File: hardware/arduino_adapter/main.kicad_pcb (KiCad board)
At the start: 2 copper layers, 65.5 x 62.5 mm, 15 parts, among them P1 CONN_8, P10 CONN_10, P11 CONN_8, P2 CONN_6, P3 CONN_6, P4 CONN_8, P5 POW, P6 TWI, P7 TWI_POW, P8 CONN_10, P9 CONN_8

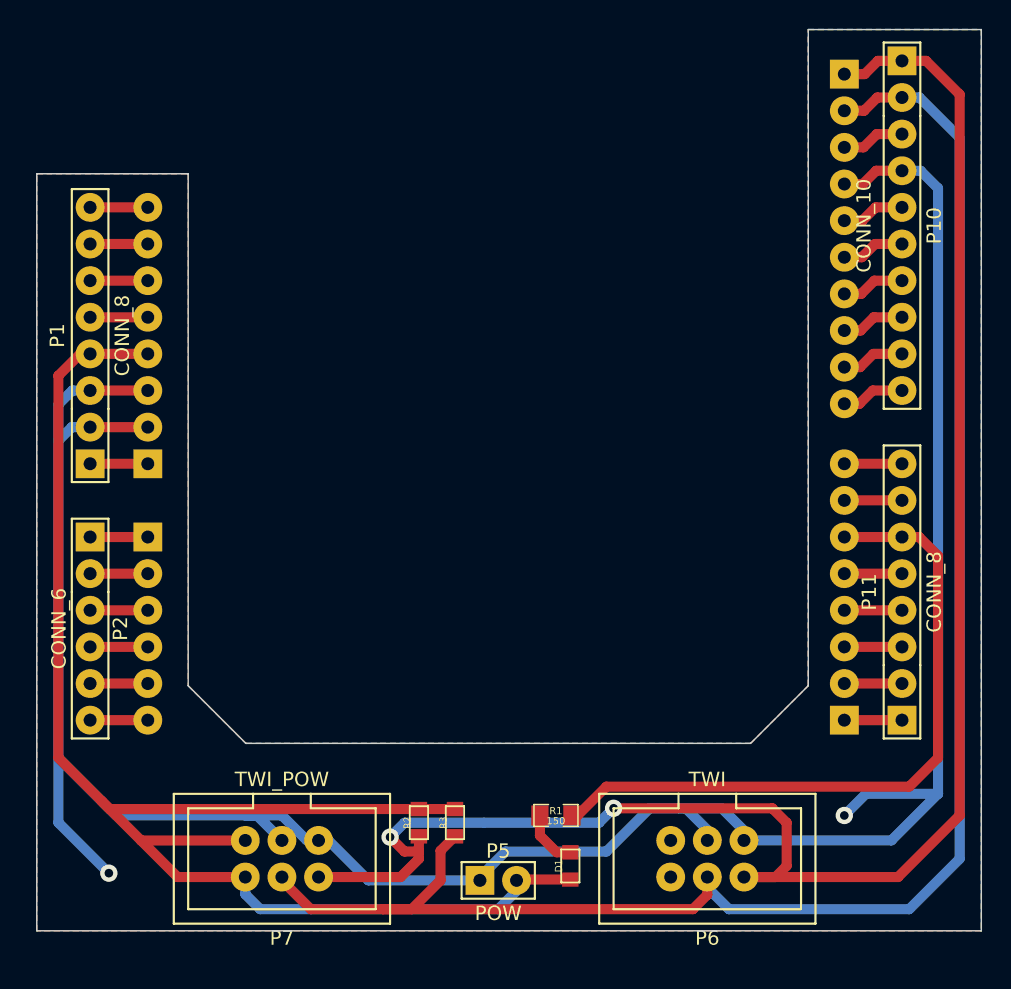
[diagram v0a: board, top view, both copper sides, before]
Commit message: modify
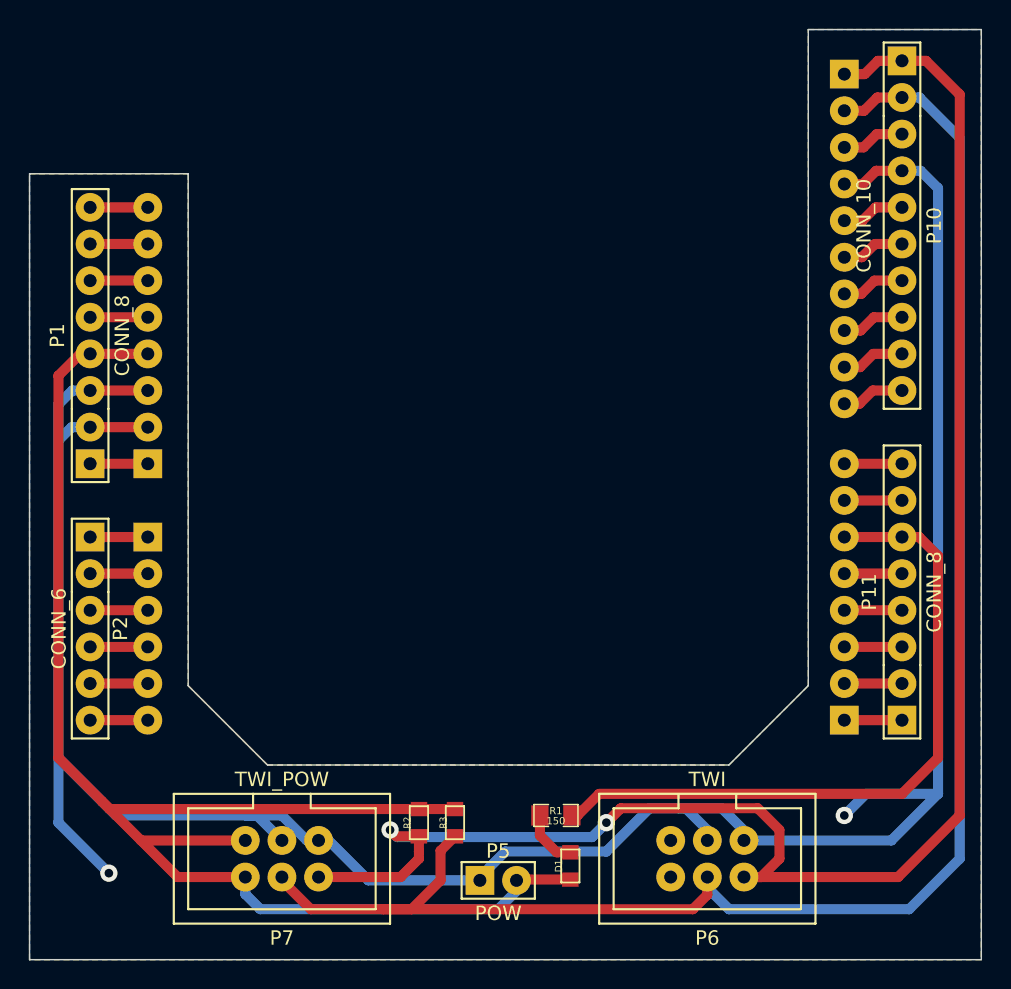
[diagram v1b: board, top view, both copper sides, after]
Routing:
- net /SCL: track 122.6 -> 120.9 mm
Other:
- board size 65.5 x 62.5 mm -> 66 x 64.5 mm
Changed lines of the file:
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@@
     (links 53)
     (no_connects 0)
-    (area 0 0 0 0)
+    (area 20.269999 46.949999 144.05 183.990001)
     (thickness 1.6)
-    (drawings 19)
-    (tracks 157)
+    (drawings 22)
+    (tracks 158)
     (zones 0)
     (modules 15)
@@
     (visible_elements FFFFFFBF)
     (pcbplotparams
-      (layerselection 3178497)
-      (usegerberextensions true)
-      (excludeedgelayer true)
+      (layerselection 32768)
+      (usegerberextensions false)
+      (excludeedgelayer false)
       (linewidth 0.150000)
       (plotframeref false)
@@
       (padsonsilk false)
       (subtractmaskfromsilk false)
-      (outputformat 1)
+      (outputformat 2)
       (mirror false)
-      (drillshape 1)
+      (drillshape 2)
       (scaleselection 1)
       (outputdirectory ""))
@@
     )
   )
+  (gr_line (start 74 98) (end 106 98) (angle 90) (layer Edge.Cuts) (width 0.1))
+  (gr_line (start 68.5 92.5) (end 74 98) (angle 90) (layer Edge.Cuts) (width 0.1))
+  (gr_line (start 68.5 57) (end 68.5 92.5) (angle 90) (layer Edge.Cuts) (width 0.1))
+  (gr_line (start 57.5 57) (end 68.5 57) (angle 90) (layer Edge.Cuts) (width 0.1))
+  (gr_line (start 57.5 111.5) (end 57.5 57) (angle 90) (layer Edge.Cuts) (width 0.1))
+  (gr_line (start 123.5 111.5) (end 57.5 111.5) (angle 90) (layer Edge.Cuts) (width 0.1))
+  (gr_line (start 123.5 47) (end 123.5 111.5) (angle 90) (layer Edge.Cuts) (width 0.1))
+  (gr_line (start 111.5 47) (end 123.5 47) (angle 90) (layer Edge.Cuts) (width 0.1))
   (gr_line (start 111.5 92.5) (end 111.5 47) (angle 90) (layer Edge.Cuts) (width 0.1))
-  (gr_line (start 107.5 96.5) (end 111.5 92.5) (angle 90) (layer Edge.Cuts) (width 0.1))
-  (gr_line (start 72.5 96.5) (end 107.5 96.5) (angle 90) (layer Edge.Cuts) (width 0.1))
-  (gr_line (start 68.5 92.5) (end 72.5 96.5) (angle 90) (layer Edge.Cuts) (width 0.1))
-  (gr_line (start 68.5 57) (end 68.5 92.5) (angle 90) (layer Edge.Cuts) (width 0.1))
-  (gr_line (start 58 57) (end 68.5 57) (angle 90) (layer Edge.Cuts) (width 0.1))
-  (gr_line (start 58 109.5) (end 58 57) (angle 90) (layer Edge.Cuts) (width 0.1))
-  (gr_line (start 123.5 109.5) (end 58 109.5) (angle 90) (layer Edge.Cuts) (width 0.1))
-  (gr_line (start 123.5 47) (end 123.5 109.5) (angle 90) (layer Edge.Cuts) (width 0.1))
-  (gr_line (start 111.5 47) (end 123.5 47) (angle 90) (layer Edge.Cuts) (width 0.1))
+  (gr_line (start 106 98) (end 111.5 92.5) (angle 90) (layer Edge.Cuts) (width 0.1))
+  (dimension 5.5 (width 0.3) (layer Cmts.User)
+    (gr_text "5.500 mm" (at 152.349999 95.250007 270) (layer Cmts.User)
+      (effects (font (size 1.5 1.5) (thickness 0.3)))
+    )
+    (feature1 (pts (xy 68.5 98) (xy 153.699999 98.000007)))
+    (feature2 (pts (xy 68.5 92.5) (xy 153.699999 92.500007)))
+    (crossbar (pts (xy 150.999999 92.500007) (xy 150.999999 98.000007)))
+    (arrow1a (pts (xy 150.999999 98.000007) (xy 150.413579 96.873504)))
+    (arrow1b (pts (xy 150.999999 98.000007) (xy 151.586419 96.873504)))
+    (arrow2a (pts (xy 150.999999 92.500007) (xy 150.413579 93.62651)))
+    (arrow2b (pts (xy 150.999999 92.500007) (xy 151.586419 93.62651)))
+  )
+  (dimension 5.5 (width 0.3) (layer Cmts.User)
+    (gr_text "5.500 mm" (at 71.25 120.849999) (layer Cmts.User)
+      (effects (font (size 1.5 1.5) (thickness 0.3)))
+    )
+    (feature1 (pts (xy 68.5 92.5) (xy 68.5 122.199999)))
+    (feature2 (pts (xy 74 92.5) (xy 74 122.199999)))
+    (crossbar (pts (xy 74 119.499999) (xy 68.5 119.499999)))
+    (arrow1a (pts (xy 68.5 119.499999) (xy 69.626503 118.913579)))
+    (arrow1b (pts (xy 68.5 119.499999) (xy 69.626503 120.086419)))
+    (arrow2a (pts (xy 74 119.499999) (xy 72.873497 118.913579)))
+    (arrow2b (pts (xy 74 119.499999) (xy 72.873497 120.086419)))
+  )
+  (dimension 5.5 (width 0.3) (layer Cmts.User)
+    (gr_text "5.500 mm" (at 108.75 121.349999) (layer Cmts.User)
+      (effects (font (size 1.5 1.5) (thickness 0.3)))
+    )
+    (feature1 (pts (xy 106 92.5) (xy 106 122.699999)))
+    (feature2 (pts (xy 111.5 92.5) (xy 111.5 122.699999)))
+    (crossbar (pts (xy 111.5 119.999999) (xy 106 119.999999)))
+    (arrow1a (pts (xy 106 119.999999) (xy 107.126503 119.413579)))
+    (arrow1b (pts (xy 106 119.999999) (xy 107.126503 120.586419)))
+    (arrow2a (pts (xy 111.5 119.999999) (xy 110.373497 119.413579)))
+    (arrow2b (pts (xy 111.5 119.999999) (xy 110.373497 120.586419)))
+  )
   (dimension 5 (width 0.3) (layer Cmts.User)
     (gr_text "5.000 mm" (at 42.150001 97.499994 270) (layer Cmts.User)
@@
     (arrow2b (pts (xy 136.05 94.89) (xy 135.46358 93.763497)))
   )
-  (segment (start 95.108 101.5) (end 95.5 101.5) (width 0.7) (layer F.Cu) (net 1))
-  (segment (start 119.19 82.19) (end 118 82.19) (width 0.7) (layer F.Cu) (net 1))
+  (segment (start 95.108 101.5) (end 95.5 101.5) (width 0.7) (layer F.Cu) (net 1) (status C00000))
+  (segment (start 119.19 82.19) (end 118 82.19) (width 0.7) (layer F.Cu) (net 1) (status 800000))
   (segment (start 120.5 83.5) (end 119.19 82.19) (width 0.7) (layer F.Cu) (net 1))
-  (segment (start 120.5 97.5) (end 120.5 83.5) (width 0.7) (layer F.Cu) (net 1))
-  (segment (start 118.5 99.5) (end 120.5 97.5) (width 0.7) (layer F.Cu) (net 1))
-  (segment (start 97.5 99.5) (end 118.5 99.5) (width 0.7) (layer F.Cu) (net 1))
-  (segment (start 95.5 101.5) (end 97.5 99.5) (width 0.7) (layer F.Cu) (net 1))
+  (segment (start 120.5 84.69) (end 120.5 83.5) (width 0.7) (layer F.Cu) (net 1))
+  (segment (start 120.5 97.5) (end 120.5 84.69) (width 0.7) (layer F.Cu) (net 1))
+  (segment (start 118 100) (end 120.5 97.5) (width 0.7) (layer F.Cu) (net 1))
+  (segment (start 97 100) (end 118 100) (width 0.7) (layer F.Cu) (net 1))
+  (segment (start 95.5 101.5) (end 97 100) (width 0.7) (layer F.Cu) (net 1) (status 400000))
   (segment (start 114 82.19) (end 118 82.19) (width 0.7) (layer F.Cu) (net 1))
+  (segment (start 84.5 102.945) (end 82.945 102.945) (width 0.7) (layer F.Cu) (net 2) (status 400000))
+  (segment (start 108.23 105.77) (end 107.04 105.77) (width 0.7) (layer F.Cu) (net 2) (status 800000))
+  (segment (start 109.5 104.5) (end 108.23 105.77) (width 0.7) (layer F.Cu) (net 2))
+  (segment (start 109.5 102.5) (end 109.5 104.5) (width 0.7) (layer F.Cu) (net 2))
+  (segment (start 108 101) (end 109.5 102.5) (width 0.7) (layer F.Cu) (net 2))
+  (segment (start 98.5 101) (end 108 101) (width 0.7) (layer F.Cu) (net 2))
+  (segment (start 97.5 102) (end 98.5 101) (width 0.7) (layer F.Cu) (net 2))
+  (via (at 97.5 102) (size 1.2) (layers F.Cu B.Cu) (net 2))
+  (segment (start 96.5 103) (end 97.5 102) (width 0.7) (layer B.Cu) (net 2))
+  (segment (start 83 103) (end 96.5 103) (width 0.7) (layer B.Cu) (net 2))
+  (segment (start 82.5 102.5) (end 83 103) (width 0.7) (layer B.Cu) (net 2))
+  (via (at 82.5 102.5) (size 1.2) (layers F.Cu B.Cu) (net 2))
+  (segment (start 82.945 102.945) (end 82.5 102.5) (width 0.7) (layer F.Cu) (net 2))
   (segment (start 107.04 105.77) (end 117.73 105.77) (width 0.7) (layer F.Cu) (net 2))
+  (segment (start 117.73 105.77) (end 122 101.5) (width 0.7) (layer F.Cu) (net 2))
+  (segment (start 122 101.5) (end 122 51.5) (width 0.7) (layer F.Cu) (net 2))
+  (segment (start 122 51.5) (end 119.67 49.17) (width 0.7) (layer F.Cu) (net 2))
   (segment (start 119.67 49.17) (end 118 49.17) (width 0.7) (layer F.Cu) (net 2))
-  (segment (start 122 51.5) (end 119.67 49.17) (width 0.7) (layer F.Cu) (net 2))
-  (segment (start 122 101.5) (end 122 51.5) (width 0.7) (layer F.Cu) (net 2))
-  (segment (start 117.73 105.77) (end 122 101.5) (width 0.7) (layer F.Cu) (net 2))
-  (segment (start 89 102) (end 97 102) (width 0.7) (layer B.Cu) (net 2))
-  (segment (start 83.5 104) (end 82.5 103) (width 0.7) (layer F.Cu) (net 2))
-  (via (at 82.5 103) (size 1.2) (layers F.Cu B.Cu) (net 2))
-  (segment (start 82.5 103) (end 83.5 102) (width 0.7) (layer B.Cu) (net 2))
-  (segment (start 83.5 102) (end 89 102) (width 0.7) (layer B.Cu) (net 2))
-  (segment (start 84.5 104) (end 83.5 104) (width 0.7) (layer F.Cu) (net 2))
-  (segment (start 109.23 105.77) (end 107.04 105.77) (width 0.7) (layer F.Cu) (net 2))
-  (segment (start 110 105) (end 109.23 105.77) (width 0.7) (layer F.Cu) (net 2))
-  (segment (start 110 102) (end 110 105) (width 0.7) (layer F.Cu) (net 2))
-  (segment (start 109 101) (end 110 102) (width 0.7) (layer F.Cu) (net 2))
-  (segment (start 98 101) (end 109 101) (width 0.7) (layer F.Cu) (net 2))
-  (via (at 98 101) (size 1.2) (layers F.Cu B.Cu) (net 2))
-  (segment (start 97 102) (end 98 101) (width 0.7) (layer B.Cu) (net 2))
   (segment (start 77.54 105.77) (end 83.23 105.77) (width 0.7) (layer F.Cu) (net 2))
   (segment (start 84.5 104.5) (end 84.5 104) (width 0.7) (layer F.Cu) (net 2))
@@
     (polygon
       (pts
-        (xy 123.5 109.5) (xy 58 109.5) (xy 58 57) (xy 68.5 57) (xy 68.5 92.5)
-        (xy 72.5 96.5) (xy 107.5 96.5) (xy 111.5 92.5) (xy 111.5 47) (xy 123.5 47)
+        (xy 123.5 111.5) (xy 57.5 111.5) (xy 57.5 57) (xy 68.5 57) (xy 68.5 92.5)
+        (xy 74 98) (xy 106 98) (xy 111.5 92.5) (xy 111.5 47) (xy 123.5 47)
       )
     )
@@
     (polygon
       (pts
-        (xy 123.5 109.5) (xy 58 109.5) (xy 58 57) (xy 68.5 57) (xy 68.5 92.5)
-        (xy 72.5 96.5) (xy 107.5 96.5) (xy 111.5 92.5) (xy 111.5 47) (xy 123.5 47)
+        (xy 123.5 111.5) (xy 57.5 111.5) (xy 57.5 57) (xy 68.5 57) (xy 68.5 92.5)
+        (xy 74 98) (xy 106 98) (xy 111.5 92.5) (xy 111.5 47) (xy 123.5 47)
       )
     )

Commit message: moved modules
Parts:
- moved D1 226.0 mm to (290.6, 218.3)
- moved P1 226.0 mm to (257.3, 181.5)
- moved P10 226.0 mm to (313.6, 173.9)
- moved P11 226.0 mm to (313.6, 199.3)
- moved P2 226.0 mm to (257.3, 201.8)
- moved P3 226.0 mm to (261.3, 201.8)
- moved P4 226.0 mm to (261.3, 181.5)
- moved P5 226.0 mm to (285.6, 219.3)
- moved P6 226.0 mm to (300.1, 217.8)
- moved P7 226.0 mm to (270.6, 217.8)
- moved P8 226.0 mm to (309.6, 174.8)
- moved P9 226.0 mm to (309.6, 199.3)
- moved R1 226.0 mm to (289.6, 214.8)
- moved R2 226.0 mm to (280.1, 215.3)
- moved R3 226.0 mm to (282.6, 215.3)
